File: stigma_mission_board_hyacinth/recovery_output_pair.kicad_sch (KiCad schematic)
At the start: 13 parts, among them Q5 AON7544, Q6 AON7544

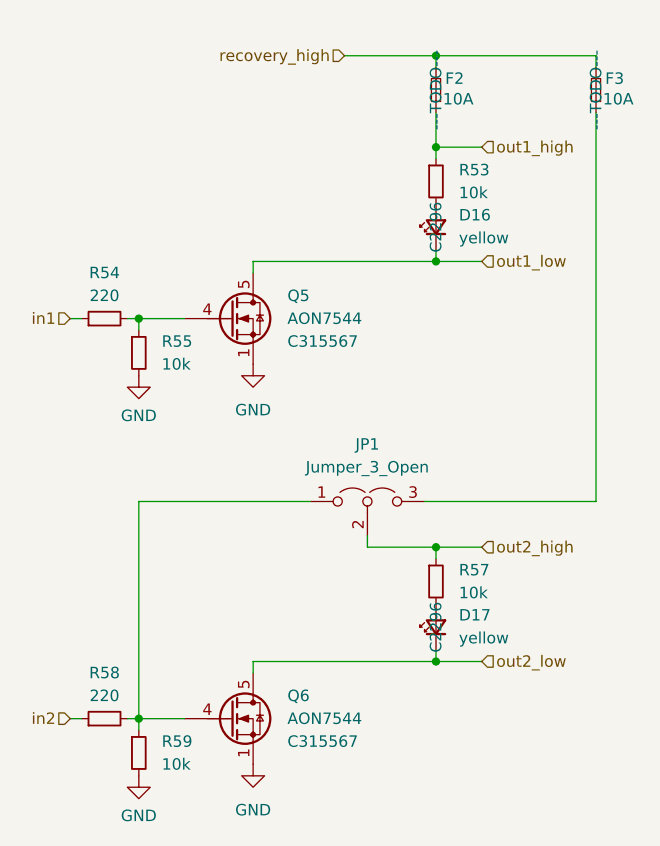
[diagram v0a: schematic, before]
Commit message: Last minute changes to mission board
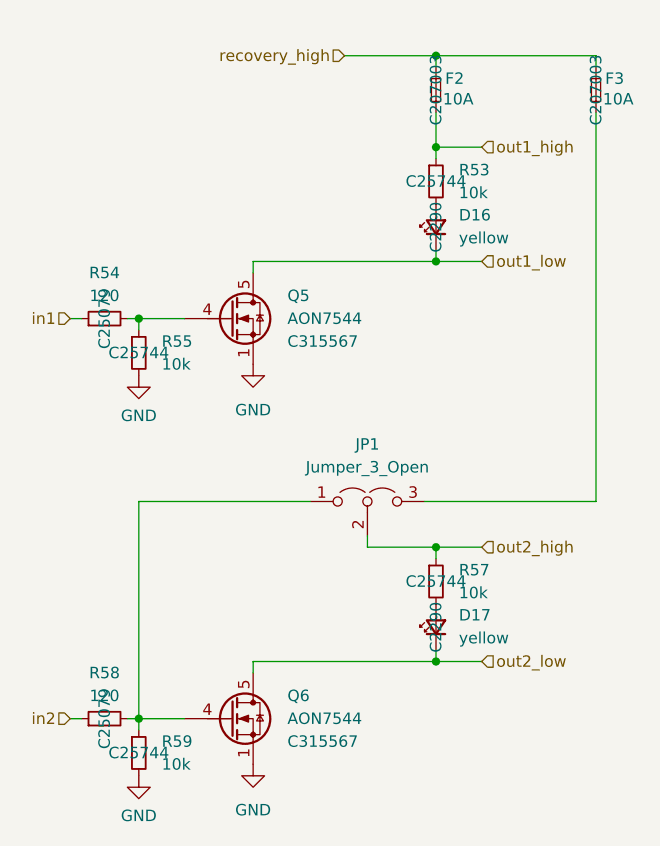
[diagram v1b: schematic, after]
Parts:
- D16, D17: LCSC C2296 -> C2290
- F2, F3: LCSC ---TODO--- -> C207003
- R53, R55, R57, R59: LCSC (none) -> C25744
- R54, R58: value 220 -> 120; LCSC (none) -> C25079
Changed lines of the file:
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@@
 			)
 		)
-		(property "LCSC" "---TODO---"
+		(property "LCSC" "C207003"
 			(at 124.46 22.86 0)
 			(effects
@@
 			)
 		)
-		(property "Value" "220"
+		(property "Value" "120"
 			(at 69.85 90.17 90)
 			(effects
@@
 			)
 		)
+		(property "LCSC" "C25079"
+			(at 69.85 92.71 0)
+			(effects
+				(font
+					(size 1.27 1.27)
+				)
+			)
+		)
 		(pin "2"
 		)
@@
 				)
 				(hide yes)
+			)
+		)
+		(property "LCSC" "C25744"
+			(at 73.66 52.07 0)
+			(effects
+				(font
+					(size 1.27 1.27)
+				)
 			)
 		)
@@
 			)
 		)
-		(property "LCSC" "---TODO---"
+		(property "LCSC" "C207003"
 			(at 106.68 22.86 0)
 			(effects
@@
 			)
 		)
+		(property "LCSC" "C25744"
+			(at 106.68 77.47 0)
+			(effects
+				(font
+					(size 1.27 1.27)
+				)
+			)
+		)
 		(pin "2"
 		)
@@
 			)
 		)
+		(property "LCSC" "C25744"
+			(at 73.66 96.52 0)
+			(effects
+				(font
+					(size 1.27 1.27)
+				)
+			)
+		)
 		(pin "2"
 		)
@@
 			)
 		)
-		(property "Value" "220"
+		(property "Value" "120"
 			(at 69.85 45.72 90)
 			(effects
@@
 			)
 		)
+		(property "LCSC" "C25079"
+			(at 69.85 48.26 0)
+			(effects
+				(font
+					(size 1.27 1.27)
+				)
+			)
+		)
 		(pin "2"
 		)
@@
 			)
 		)
+		(property "LCSC" "C25744"
+			(at 106.68 33.02 0)
+			(effects
+				(font
+					(size 1.27 1.27)
+				)
+			)
+		)
 		(pin "2"
 		)
@@
 			)
 		)
-		(property "LCSC" "C2296"
+		(property "LCSC" "C2290"
 			(at 106.68 38.1 0)
 			(effects
@@
 			)
 		)
-		(property "LCSC" "C2296"
+		(property "LCSC" "C2290"
 			(at 106.68 82.55 0)
 			(effects
